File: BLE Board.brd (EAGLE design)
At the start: 51.3 x 67 mm, 38 parts, among them IC1 TM4C123GH6PM, IC2 TPS6300

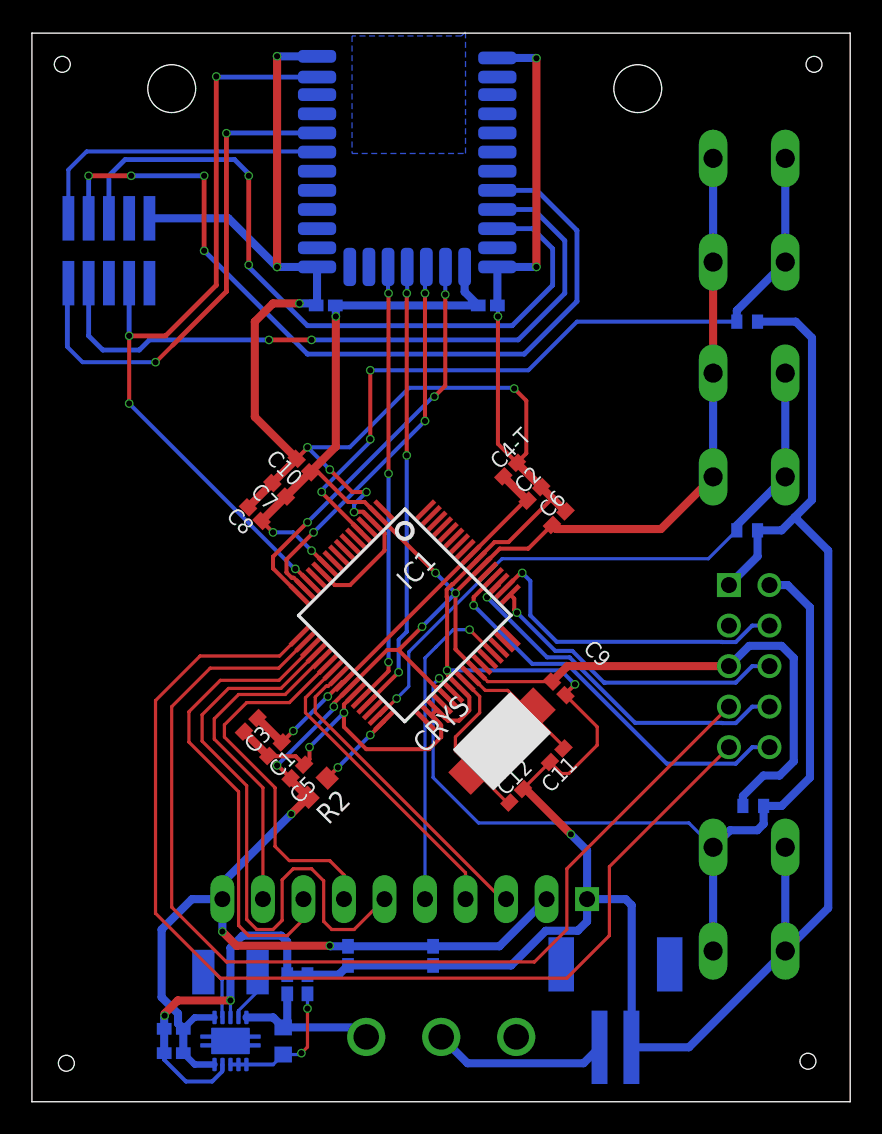
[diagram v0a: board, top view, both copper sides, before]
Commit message: Fix all errors
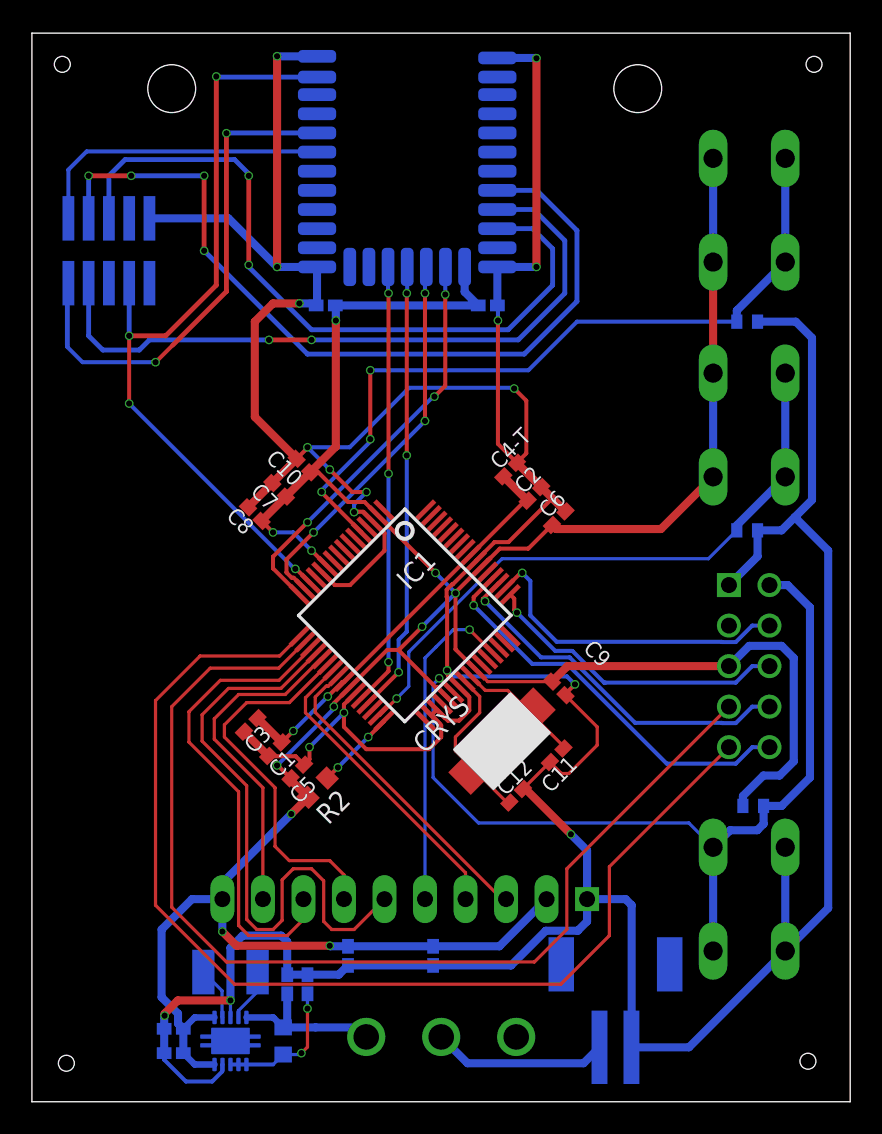
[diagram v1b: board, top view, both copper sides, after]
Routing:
- net N$4: track 3.92 -> 3.34 mm
- removed copper zone on layer 16, net N$2
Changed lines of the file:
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@@
 <hole x="-3.429" y="2.413" drill="1"/>
 <hole x="43.053" y="2.54" drill="1"/>
+<polygon width="0.4064" layer="39">
+<vertex x="14.859" y="65.659"/>
+<vertex x="14.859" y="59.944"/>
+<vertex x="14.986" y="59.817"/>
+<vertex x="21.082" y="59.817"/>
+<vertex x="21.082" y="65.532"/>
+<vertex x="20.955" y="65.659"/>
+</polygon>
 </plain>
 <attributes>
@@
 <wire x1="22.98839375" y1="26.3322625" x2="22.437828125" y2="26.882828125" width="0.2032" layer="1"/>
 <wire x1="22.437828125" y1="26.882828125" x2="22.270125" y2="27.05053125" width="0.2032" layer="1"/>
-<wire x1="22.270125" y1="27.05053125" x2="22.134359375" y2="27.05053125" width="0.2032" layer="1"/>
 <wire x1="6.35" y1="12.7" x2="6.35" y2="13.716" width="0.508" layer="16"/>
 <wire x1="6.35" y1="13.716" x2="10.668" y2="18.034" width="0.508" layer="16"/>
@@
 <wire x1="22.387" y1="49.911" x2="13.427" y2="49.911" width="0.508" layer="16"/>
 <wire x1="13.427" y1="49.911" x2="13.462" y2="49.876" width="0.508" layer="16"/>
-<wire x1="13.462" y1="49.876" x2="13.462" y2="49.2208" width="0.508" layer="16"/>
-<via x="13.462" y="49.2208" extent="1-16" drill="0.381" diameter="0.55"/>
-<wire x1="13.462" y1="49.2208" x2="13.462" y2="41.061471875" width="0.508" layer="1"/>
+<wire x1="13.462" y1="49.876" x2="13.462" y2="48.9668" width="0.508" layer="16"/>
+<via x="13.462" y="48.9668" extent="1-16" drill="0.381" diameter="0.55"/>
+<wire x1="13.462" y1="48.9668" x2="13.462" y2="41.061471875" width="0.508" layer="1"/>
 <wire x1="13.462" y1="41.061471875" x2="11.8542625" y2="39.453734375" width="0.508" layer="1"/>
 <wire x1="21.534" y1="52.324" x2="21.534" y2="50.764" width="0.508" layer="16"/>
@@
 <wire x1="27.8562625" y1="25.5702625" x2="28.448" y2="26.162" width="0.254" layer="1"/>
 <via x="28.448" y="26.162" extent="1-16" drill="0.381" diameter="0.55"/>
-<wire x1="28.448" y1="26.162" x2="27.570328125" y2="27.039671875" width="0.254" layer="16"/>
-<wire x1="27.570328125" y1="27.039671875" x2="20.435671875" y2="27.039671875" width="0.254" layer="16"/>
+<wire x1="28.448" y1="26.162" x2="27.951328125" y2="26.658671875" width="0.254" layer="16"/>
+<wire x1="27.951328125" y1="26.658671875" x2="20.816671875" y2="26.658671875" width="0.254" layer="16"/>
+<wire x1="20.816671875" y1="26.658671875" x2="20.435671875" y2="27.039671875" width="0.254" layer="16"/>
 <via x="20.435671875" y="27.039671875" extent="1-16" drill="0.381" diameter="0.55"/>
 <wire x1="20.435671875" y1="27.039671875" x2="20.435671875" y2="26.830371875" width="0.254" layer="1"/>
@@
 <wire x1="8.382" y1="48.895" x2="9.525" y2="50.038" width="0.508" layer="1"/>
 <wire x1="23.587" y1="49.911" x2="23.622" y2="49.876" width="0.254" layer="16"/>
-<wire x1="23.622" y1="49.876" x2="23.622" y2="49.2208" width="0.254" layer="16"/>
-<via x="23.622" y="49.2208" extent="1-16" drill="0.381" diameter="0.55"/>
-<wire x1="23.622" y1="49.2208" x2="23.622" y2="41.234525" width="0.254" layer="1"/>
+<wire x1="23.622" y1="49.876" x2="23.622" y2="48.9668" width="0.254" layer="16"/>
+<via x="23.622" y="48.9668" extent="1-16" drill="0.381" diameter="0.55"/>
+<wire x1="23.622" y1="48.9668" x2="23.622" y2="41.234525" width="0.254" layer="1"/>
 <wire x1="23.622" y1="41.234525" x2="24.8082625" y2="40.0482625" width="0.254" layer="1"/>
 <wire x1="11.005734375" y1="40.3022625" x2="11.684" y2="40.980528125" width="0.254" layer="1"/>
@@
 <wire x1="39.56145" y1="24.765" x2="38.52805" y2="23.7316" width="0.254" layer="16"/>
 <wire x1="37.67195" y1="23.7316" x2="37.65455" y2="23.749" width="0.254" layer="16"/>
-<via x="22.938740625" y="31.623" extent="1-16" drill="0.381" diameter="0.55"/>
+<via x="22.811740625" y="31.369" extent="1-16" drill="0.381" diameter="0.55"/>
 <wire x1="32.21978125" y1="23.749" x2="28.11630625" y2="27.852475" width="0.254" layer="16"/>
-<wire x1="26.709265625" y1="27.852475" x2="22.938740625" y2="31.623" width="0.254" layer="16"/>
-<wire x1="28.11630625" y1="27.852475" x2="26.709265625" y2="27.852475" width="0.254" layer="16"/>
-<wire x1="22.938740625" y1="31.623" x2="23.08674375" y2="31.771003125" width="0.254" layer="1"/>
-<wire x1="23.08674375" y1="31.771003125" x2="23.08674375" y2="31.7978125" width="0.254" layer="1"/>
-<wire x1="23.08674375" y1="31.7978125" x2="23.684340625" y2="32.395409375" width="0.254" layer="1"/>
-<wire x1="23.684340625" y1="32.395409375" x2="23.684340625" y2="32.495253125" width="0.254" layer="1"/>
+<wire x1="26.328265625" y1="27.852475" x2="22.811740625" y2="31.369" width="0.254" layer="16"/>
+<wire x1="28.11630625" y1="27.852475" x2="26.328265625" y2="27.852475" width="0.254" layer="16"/>
+<wire x1="22.811740625" y1="31.369" x2="22.6713375" y2="31.50940625" width="0.254" layer="1"/>
+<wire x1="23.684340625" y1="32.495253125" x2="23.657184375" y2="32.495253125" width="0.254" layer="1"/>
+<wire x1="23.657184375" y1="32.495253125" x2="22.6713375" y2="31.50940625" width="0.254" layer="1"/>
 <wire x1="37.65455" y1="23.749" x2="32.21978125" y2="23.749" width="0.254" layer="16"/>
 </signal>
@@
 <contactref element="IC1" pad="32"/>
 <contactref element="R2" pad="1"/>
-<wire x1="12.920040625" y1="20.316740625" x2="12.920040625" y2="20.286040625" width="0.2032" layer="1"/>
+<via x="13.589" y="20.955" extent="1-16" drill="0.381" diameter="0.55"/>
 <wire x1="12.920040625" y1="20.286040625" x2="13.589" y2="20.955" width="0.254" layer="1"/>
-<via x="13.589" y="20.955" extent="1-16" drill="0.381" diameter="0.55"/>
-<wire x1="13.589" y1="20.955" x2="15.621" y2="22.987" width="0.254" layer="16"/>
-<via x="15.621" y="22.987" extent="1-16" drill="0.381" diameter="0.55"/>
-<wire x1="15.621" y1="22.987" x2="16.47185" y2="23.83785" width="0.254" layer="1"/>
+<wire x1="15.494" y1="22.86" x2="13.589" y2="20.955" width="0.254" layer="16"/>
+<via x="15.494" y="22.86" extent="1-16" drill="0.381" diameter="0.55"/>
+<wire x1="15.494" y1="22.86" x2="16.47185" y2="23.83785" width="0.254" layer="1"/>
 <wire x1="16.47185" y1="23.83785" x2="16.47185" y2="23.86855" width="0.254" layer="1"/>
 </signal>
@@
 <contactref element="IC2" pad="5"/>
 <contactref element="ON/OFF" pad="P$1"/>
-<wire x1="7.858" y1="5.285" x2="9.535" y2="5.285" width="0.508" layer="16"/>
-<wire x1="9.535" y1="5.285" x2="10.16" y2="4.66" width="0.508" layer="16"/>
-<wire x1="10.16" y1="4.66" x2="14.77" y2="4.66" width="0.508" layer="16"/>
+<wire x1="10.16" y1="4.66" x2="12.192" y2="4.66" width="0.508" layer="16"/>
+<wire x1="12.192" y1="4.66" x2="14.77" y2="4.66" width="0.508" layer="16"/>
 <wire x1="14.77" y1="4.66" x2="15.366" y2="4.064" width="0.508" layer="16"/>
 <wire x1="10.414" y1="6.766" x2="10.414" y2="4.914" width="0.508" layer="16"/>
 <wire x1="10.414" y1="4.914" x2="10.16" y2="4.66" width="0.508" layer="16"/>
+<wire x1="10.16" y1="4.66" x2="9.535" y2="5.285" width="0.4064" layer="16"/>
+<wire x1="9.535" y1="5.285" x2="7.858" y2="5.285" width="0.4064" layer="16"/>
 </signal>
 <signal name="N$1">
@@
 <contactref element="L1" pad="2"/>
 <contactref element="IC2" pad="2"/>
-<wire x1="6.329" y1="7.641" x2="5.842" y2="8.128" width="0.2032" layer="16"/>
-<wire x1="5.842" y1="8.128" x2="5.715" y2="8.255" width="0.2032" layer="16"/>
-<wire x1="6.329" y1="7.641" x2="6.329" y2="5.314" width="0.2032" layer="16"/>
+<wire x1="5.158" y1="8.128" x2="6.329" y2="6.957" width="0.2032" layer="16"/>
+<wire x1="6.329" y1="6.957" x2="6.329" y2="5.314" width="0.2032" layer="16"/>
 <wire x1="6.329" y1="5.314" x2="6.358" y2="5.285" width="0.2032" layer="16"/>
-<wire x1="5.158" y1="8.128" x2="5.842" y2="8.128" width="0.2032" layer="16"/>
 </signal>
 <signal name="MISO">
@@
 <wire x1="25.794" y1="54.724" x2="27.051" y2="53.467" width="0.3048" layer="16"/>
 <wire x1="27.051" y1="53.467" x2="27.051" y2="51.181" width="0.3048" layer="16"/>
-<wire x1="27.051" y1="51.181" x2="24.511" y2="48.641" width="0.3048" layer="16"/>
-<wire x1="24.511" y1="48.641" x2="11.684" y2="48.641" width="0.3048" layer="16"/>
-<wire x1="11.684" y1="48.641" x2="8.001" y2="52.324" width="0.3048" layer="16"/>
+<wire x1="27.051" y1="51.181" x2="24.257" y2="48.387" width="0.3048" layer="16"/>
+<wire x1="24.257" y1="48.387" x2="11.938" y2="48.387" width="0.3048" layer="16"/>
+<wire x1="11.938" y1="48.387" x2="8.001" y2="52.324" width="0.3048" layer="16"/>
 <wire x1="8.001" y1="52.324" x2="8.001" y2="52.451" width="0.3048" layer="16"/>
 <wire x1="8.001" y1="58.039" x2="8.001" y2="58.166" width="0.3048" layer="16"/>
@@
 <wire x1="38.1" y1="22.225" x2="30.607" y2="14.732" width="0.2032" layer="1"/>
 <wire x1="30.607" y1="14.732" x2="30.607" y2="10.414" width="0.2032" layer="1"/>
-<wire x1="30.607" y1="10.414" x2="27.94" y2="7.747" width="0.2032" layer="1"/>
-<wire x1="27.94" y1="7.747" x2="6.223" y2="7.747" width="0.2032" layer="1"/>
-<wire x1="6.223" y1="7.747" x2="2.159" y2="11.811" width="0.2032" layer="1"/>
-<wire x1="2.159" y1="11.811" x2="2.159" y2="25.146" width="0.2032" layer="1"/>
+<wire x1="30.607" y1="10.414" x2="27.559" y2="7.366" width="0.2032" layer="1"/>
+<wire x1="27.559" y1="7.366" x2="7.112" y2="7.366" width="0.2032" layer="1"/>
+<wire x1="7.112" y1="7.366" x2="2.159" y2="12.319" width="0.2032" layer="1"/>
+<wire x1="2.159" y1="12.319" x2="2.159" y2="25.146" width="0.2032" layer="1"/>
 <wire x1="9.9367" y1="27.94" x2="11.16855" y2="29.17185" width="0.2032" layer="1"/>
 <wire x1="2.159" y1="25.146" x2="4.953" y2="27.94" width="0.2032" layer="1"/>
 <wire x1="4.953" y1="27.94" x2="9.9367" y2="27.94" width="0.2032" layer="1"/>
 </signal>
-<signal name="N$2">
-<polygon width="0.1524" layer="16">
-<vertex x="14.478" y="66.802"/>
-<vertex x="14.478" y="59.436"/>
-<vertex x="21.59" y="59.436"/>
-<vertex x="21.59" y="67.056"/>
-<vertex x="21.336" y="66.802"/>
-</polygon>
-</signal>
 </signals>
